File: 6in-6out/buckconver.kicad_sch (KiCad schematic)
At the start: 14 parts, among them J22 Screw_Terminal_01x02, U3 MP2451DJ-LF-P

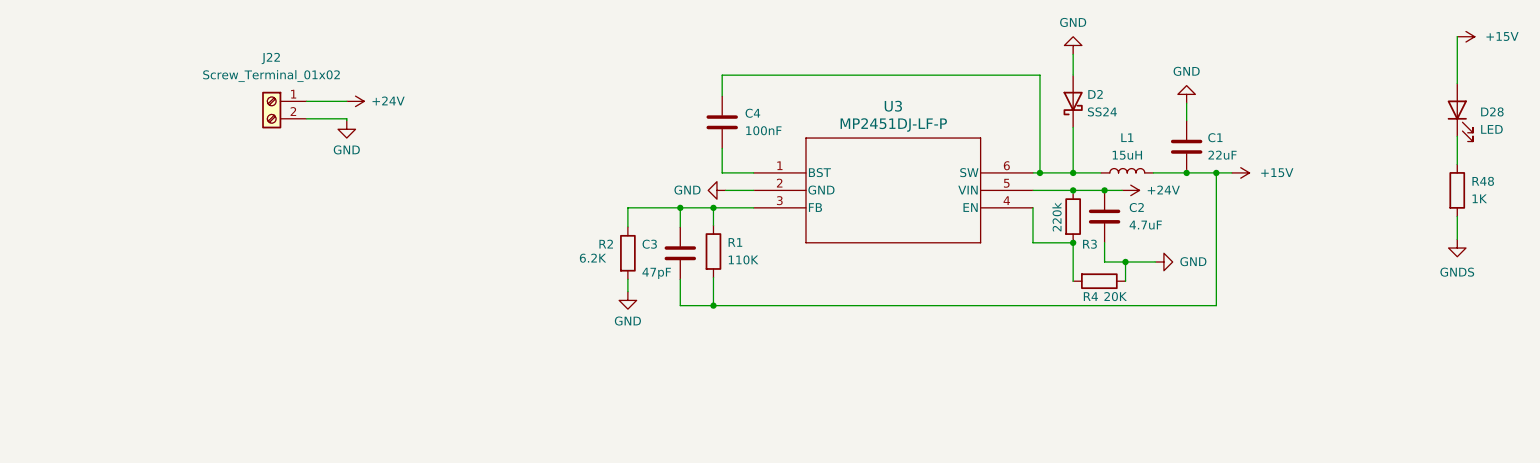
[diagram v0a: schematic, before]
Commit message: no message
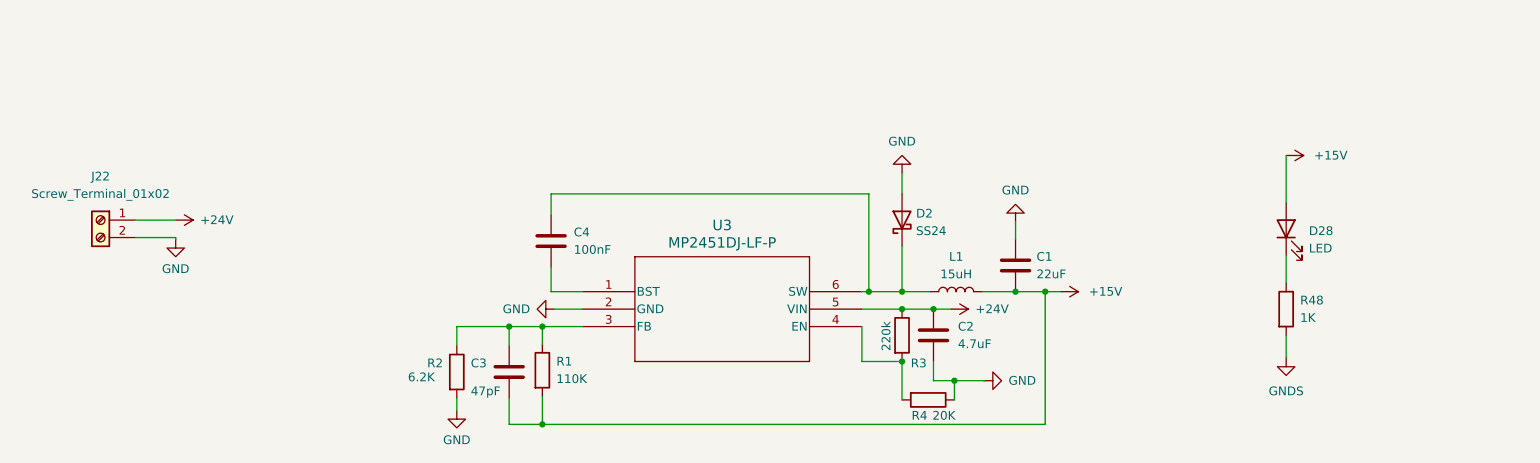
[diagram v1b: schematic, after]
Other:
- moved on the sheet: C1, C2, C3, C4, D2, D28, J22, L1, R1, R2, R3, R4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
